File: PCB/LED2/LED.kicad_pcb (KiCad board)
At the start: 2 copper layers, 70 x 70 mm, 28 parts, among them J1 Conn_01x03, J2 USB-C, U1 ESP32-PICO-MINI-02, U2 QR, U3 MD8942, U4 Barcode, U5 CH340X

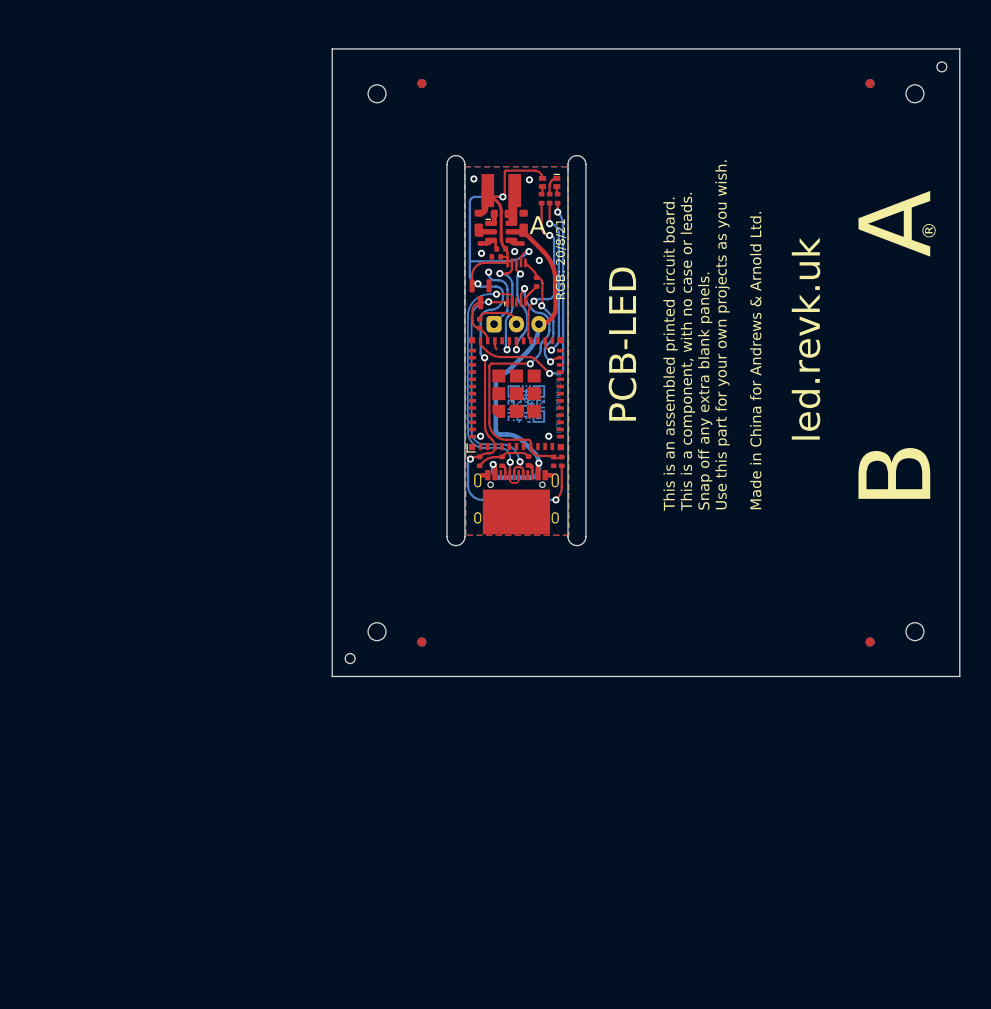
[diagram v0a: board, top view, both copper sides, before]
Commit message: VCUT
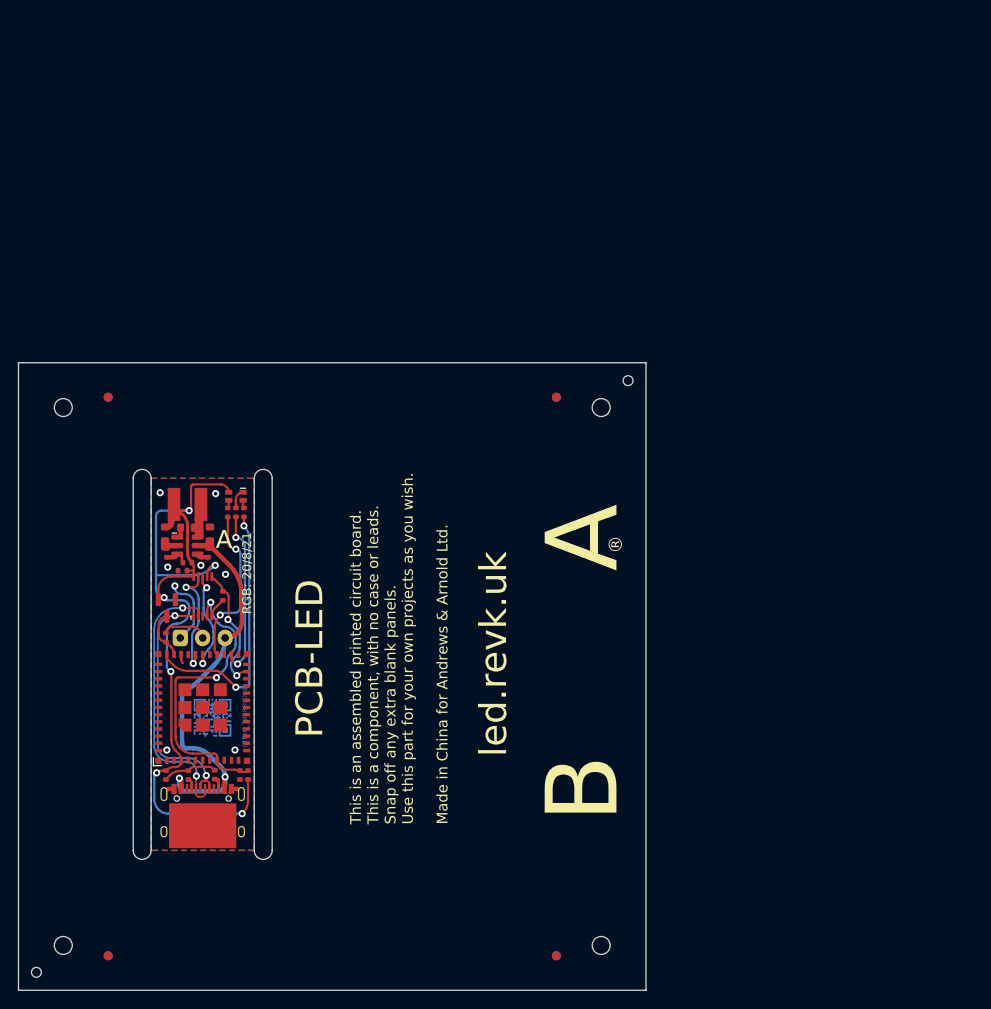
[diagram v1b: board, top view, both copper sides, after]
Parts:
- added V1: ~, RevK:VCUT70, F.Cu at (100.0, 77.9)
- added V2: ~, RevK:VCUT70, F.Cu at (100.0, 119.4)
- moved C4 49.5 mm to (83.8, 83.4)
- moved D2 49.5 mm to (89.2, 79.9)
- moved R7 49.5 mm to (81.5, 95.7)
- moved U3 49.5 mm to (83.8, 85.4)
- moved U4 49.5 mm to (105.4, 80.0)
- moved C1 49.5 mm to (89.7, 111.0)
- moved C5 49.5 mm to (81.5, 111.0)
- moved C6 49.5 mm to (83.3, 88.2)
- moved D3 49.5 mm to (81.5, 92.4)
- moved J1 49.5 mm to (85.5, 95.7)
- moved J2 49.5 mm to (85.5, 115.0)
- moved L1 49.5 mm to (83.8, 80.8)
- moved PCB1 49.5 mm to (100.0, 100.0)
- moved R1 49.5 mm to (90.6, 111.0)
- moved R10 49.5 mm to (81.5, 86.2)
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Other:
- board text added: "${TITLE}"
- board text removed: "PCB-LED"
